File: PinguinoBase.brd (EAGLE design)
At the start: 96.5 x 68.6 mm, 27 parts, among them IC1 7805, Q1 20MHz, X1 

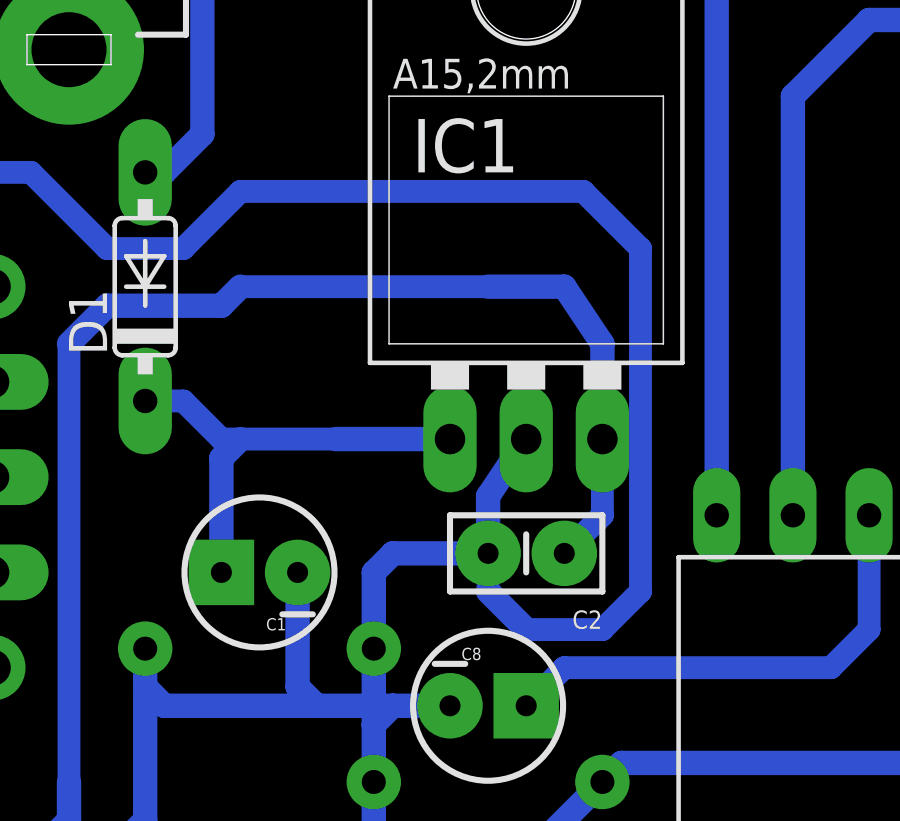
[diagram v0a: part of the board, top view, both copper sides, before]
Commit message: Fix
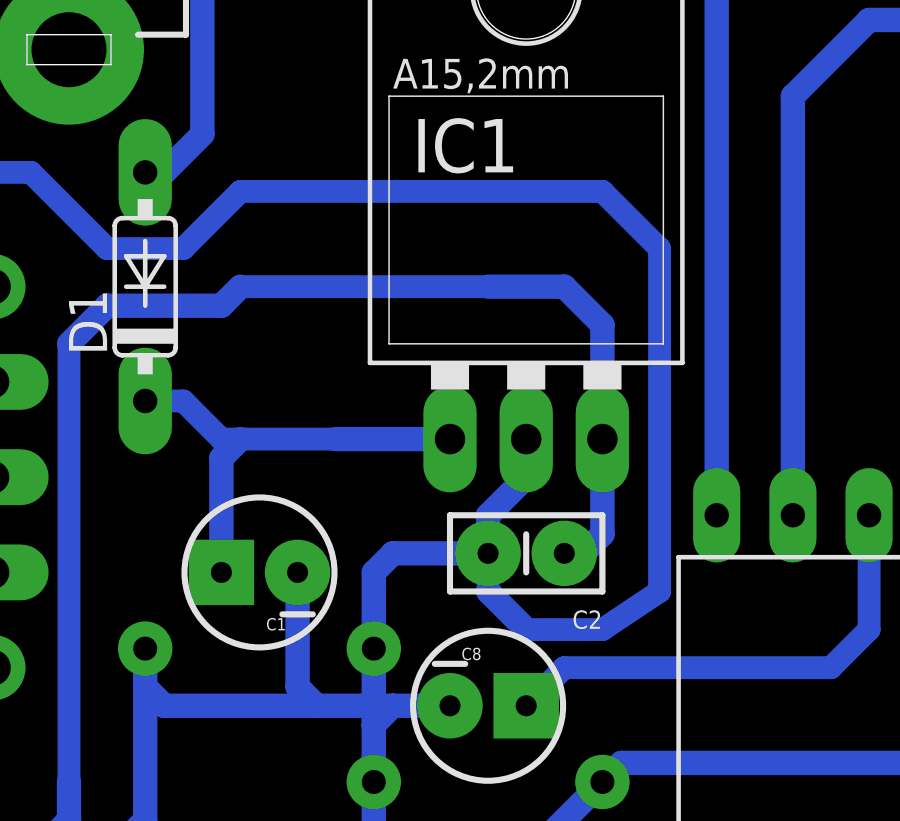
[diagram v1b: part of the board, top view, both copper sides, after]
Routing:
- net GND: track 329.7 -> 330.9 mm
- net N$3: track 49.2 -> 49.7 mm
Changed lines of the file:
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@@
 <wire x1="59.69" y1="29.21" x2="59.69" y2="26.67" width="0.762" layer="16"/>
 <wire x1="18.415" y1="52.705" x2="16.51" y2="50.8" width="0.762" layer="16"/>
-<wire x1="31.75" y1="50.8" x2="29.845" y2="52.705" width="0.762" layer="16"/>
-<wire x1="29.845" y1="52.705" x2="18.415" y2="52.705" width="0.762" layer="16"/>
-<wire x1="30.48" y1="38.1" x2="31.75" y2="39.37" width="0.762" layer="16"/>
-<wire x1="31.75" y1="39.37" x2="31.75" y2="50.8" width="0.762" layer="16"/>
+<wire x1="32.385" y1="50.8" x2="30.48" y2="52.705" width="0.762" layer="16"/>
+<wire x1="30.48" y1="52.705" x2="18.415" y2="52.705" width="0.762" layer="16"/>
+<wire x1="30.48" y1="38.1" x2="32.385" y2="39.37" width="0.762" layer="16"/>
+<wire x1="32.385" y1="39.37" x2="32.385" y2="50.8" width="0.762" layer="16"/>
 <wire x1="54.61" y1="64.135" x2="55.88" y2="65.405" width="0.762" layer="16"/>
 <wire x1="57.15" y1="32.385" x2="57.15" y2="31.75" width="0.762" layer="16"/>
@@
 <wire x1="90.17" y1="63.5" x2="90.17" y2="58.42" width="0.8128" layer="16"/>
 <wire x1="57.15" y1="31.75" x2="59.69" y2="29.21" width="0.8128" layer="16"/>
-<wire x1="26.67" y1="40.64" x2="26.67" y2="42.545" width="0.8128" layer="16"/>
-<wire x1="26.67" y1="42.545" x2="27.94" y2="44.45" width="0.8128" layer="16"/>
 <wire x1="22.86" y1="34.925" x2="22.86" y2="33.02" width="0.8128" layer="16"/>
 <wire x1="22.86" y1="34.925" x2="22.86" y2="37.465" width="0.8128" layer="16"/>
@@
 </polygon>
 <contactref element="X1" pad="2"/>
-<wire x1="5.08" y1="59.69" x2="9.7" y2="62.23" width="0" layer="19" extent="1-1"/>
+<wire x1="9.7" y1="62.23" x2="5.08" y2="59.69" width="0" layer="19" extent="1-1"/>
+<wire x1="26.67" y1="40.64" x2="26.67" y2="41.91" width="0.8128" layer="16"/>
+<wire x1="26.67" y1="41.91" x2="27.94" y2="43.18" width="0.8128" layer="16"/>
+<wire x1="27.94" y1="43.18" x2="27.94" y2="44.45" width="0.8128" layer="16"/>
 </signal>
 <signal name="N$2">
@@
 <contactref element="C2" pad="1"/>
 <wire x1="12.7" y1="33.02" x2="12.7" y2="47.625" width="0.762" layer="16"/>
-<wire x1="30.48" y1="44.45" x2="30.48" y2="41.91" width="0.762" layer="16"/>
-<wire x1="30.48" y1="41.91" x2="29.21" y2="40.64" width="0.762" layer="16"/>
 <wire x1="18.415" y1="49.53" x2="26.67" y2="49.53" width="0.762" layer="16"/>
 <wire x1="26.67" y1="49.53" x2="29.21" y2="49.53" width="0.8128" layer="16"/>
-<wire x1="29.21" y1="49.53" x2="30.48" y2="47.625" width="0.8128" layer="16"/>
-<wire x1="30.48" y1="47.625" x2="30.48" y2="44.45" width="0.8128" layer="16"/>
+<wire x1="29.21" y1="49.53" x2="30.48" y2="48.26" width="0.8128" layer="16"/>
+<wire x1="30.48" y1="48.26" x2="30.48" y2="44.45" width="0.8128" layer="16"/>
 <wire x1="17.78" y1="48.895" x2="18.415" y2="49.53" width="0.8128" layer="16"/>
 <wire x1="13.97" y1="48.895" x2="17.78" y2="48.895" width="0.8128" layer="16"/>
@@
 <wire x1="12.7" y1="31.75" x2="12.7" y2="33.02" width="0.8128" layer="16"/>
 <wire x1="6.985" y1="30.48" x2="11.43" y2="30.48" width="0.8128" layer="16"/>
+<wire x1="29.21" y1="40.64" x2="29.845" y2="40.64" width="0.8128" layer="16"/>
+<wire x1="29.845" y1="40.64" x2="30.48" y2="41.275" width="0.8128" layer="16"/>
+<wire x1="30.48" y1="41.275" x2="30.48" y2="44.45" width="0.8128" layer="16"/>
 </signal>
 <signal name="+5V">
